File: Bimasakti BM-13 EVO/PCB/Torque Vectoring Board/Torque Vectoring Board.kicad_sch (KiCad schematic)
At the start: 23 parts, among them U3 SN65HVD230, U4 SN65HVD230, U5 ADS1115IDGS

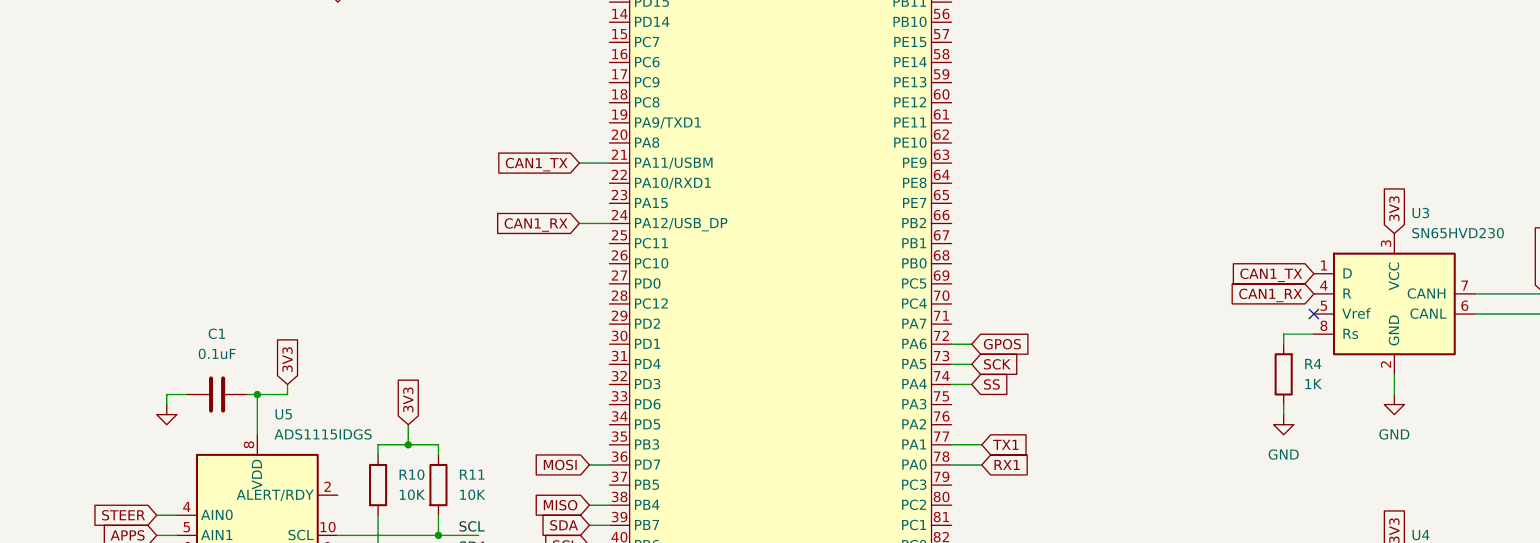
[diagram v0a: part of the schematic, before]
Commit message: cicil assembly
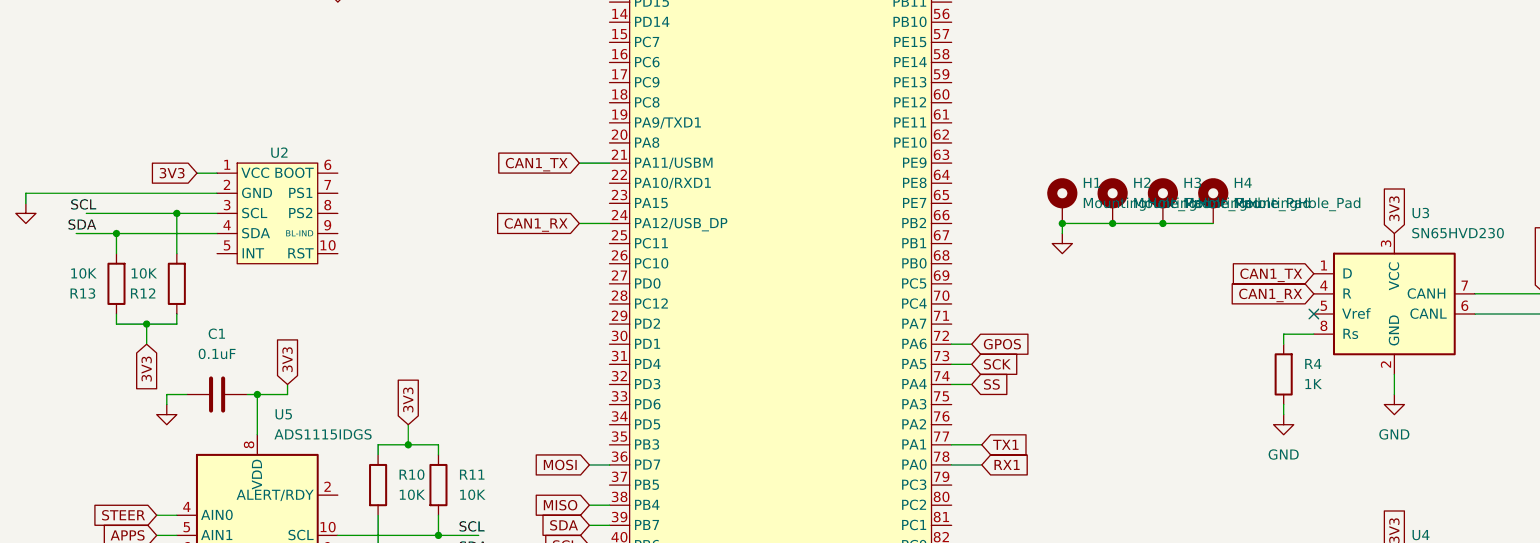
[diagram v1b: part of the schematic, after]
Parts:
- added H1, H2, H3, H4: MountingHole_Pad, MountingHole:MountingHole_3.2mm_M3_ISO7380_Pad_TopBottom, symbol Mechanical:MountingHole_Pad
- added R12, R13: 10K, Resistor_SMD:R_0805_2012Metric, symbol Device:R
- added U2: ~, 0_bno055:0_BNO055, symbol 0_BNO055:bno055
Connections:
- net 3V3: now also R12.1, R13.1, U2.1 (VCC)
- net GND: now also H1.1, H2.1, H3.1, H4.1, U2.2 (GND)
- net SCL: now also R12.2, U2.3 (SCL)
- net SDA: now also R13.2, U2.4 (SDA)
